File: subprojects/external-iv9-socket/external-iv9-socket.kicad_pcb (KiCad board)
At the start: 2 copper layers, 17.8 x 16.3 mm, 3 parts, among them J1 PINHD_1x6_Male, J3 PINHD_1x4_Male

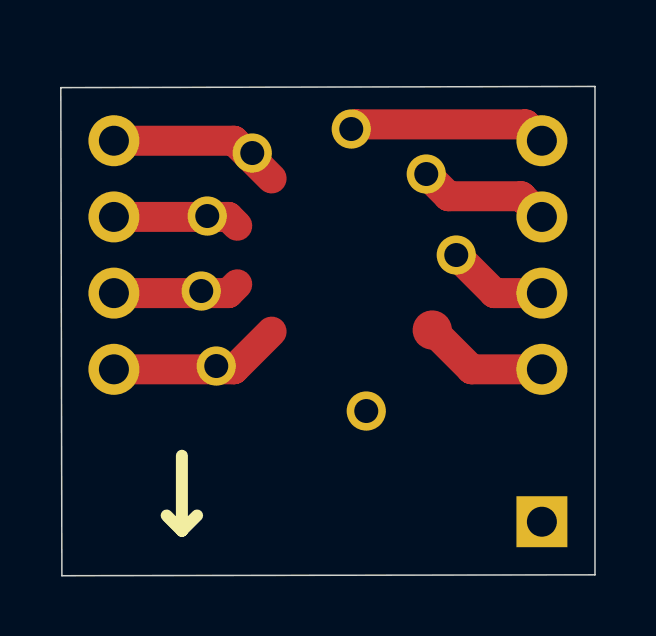
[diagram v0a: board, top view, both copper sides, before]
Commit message: Prvá iterácia.
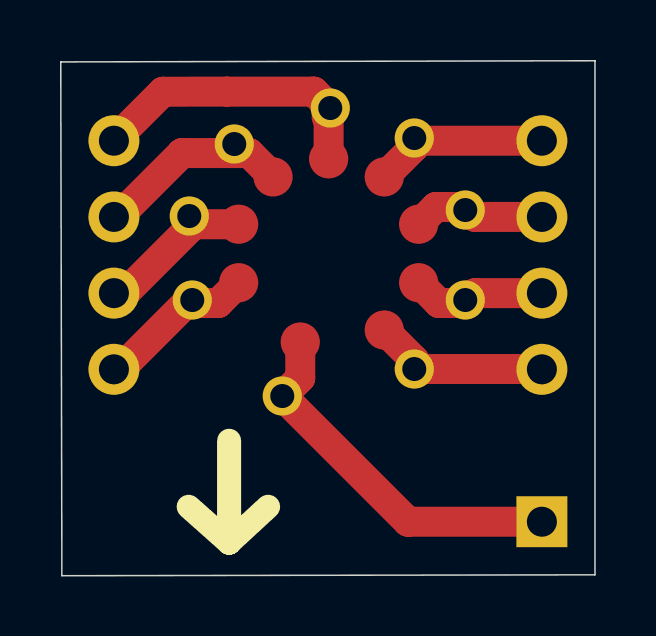
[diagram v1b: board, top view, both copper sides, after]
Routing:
- net Net-(J1-Pad1): track 0.00 -> 12.4 mm
- net Net-(J3-Pad1): track 5.78 -> 9.54 mm
- net Net-(J3-Pad2): track 4.23 -> 6.51 mm
- net Net-(J1-Pad3): track 4.20 -> 5.97 mm
- net Net-(J1-Pad4): track 3.38 -> 4.53 mm
- net Net-(J3-Pad3): track 4.23 -> 5.11 mm
- net Net-(J1-Pad6): track 6.64 -> 6.00 mm
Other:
- board size 17.8 x 16.3 mm -> 17.8 x 17.2 mm
